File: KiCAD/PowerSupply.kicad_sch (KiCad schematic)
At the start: 63 parts, among them U10 TPS7A39, U11 GM1200, U7 ADP5070ACPZ-R7, U8 TPS7A2033DQN, U9 TPS7A2033DQN

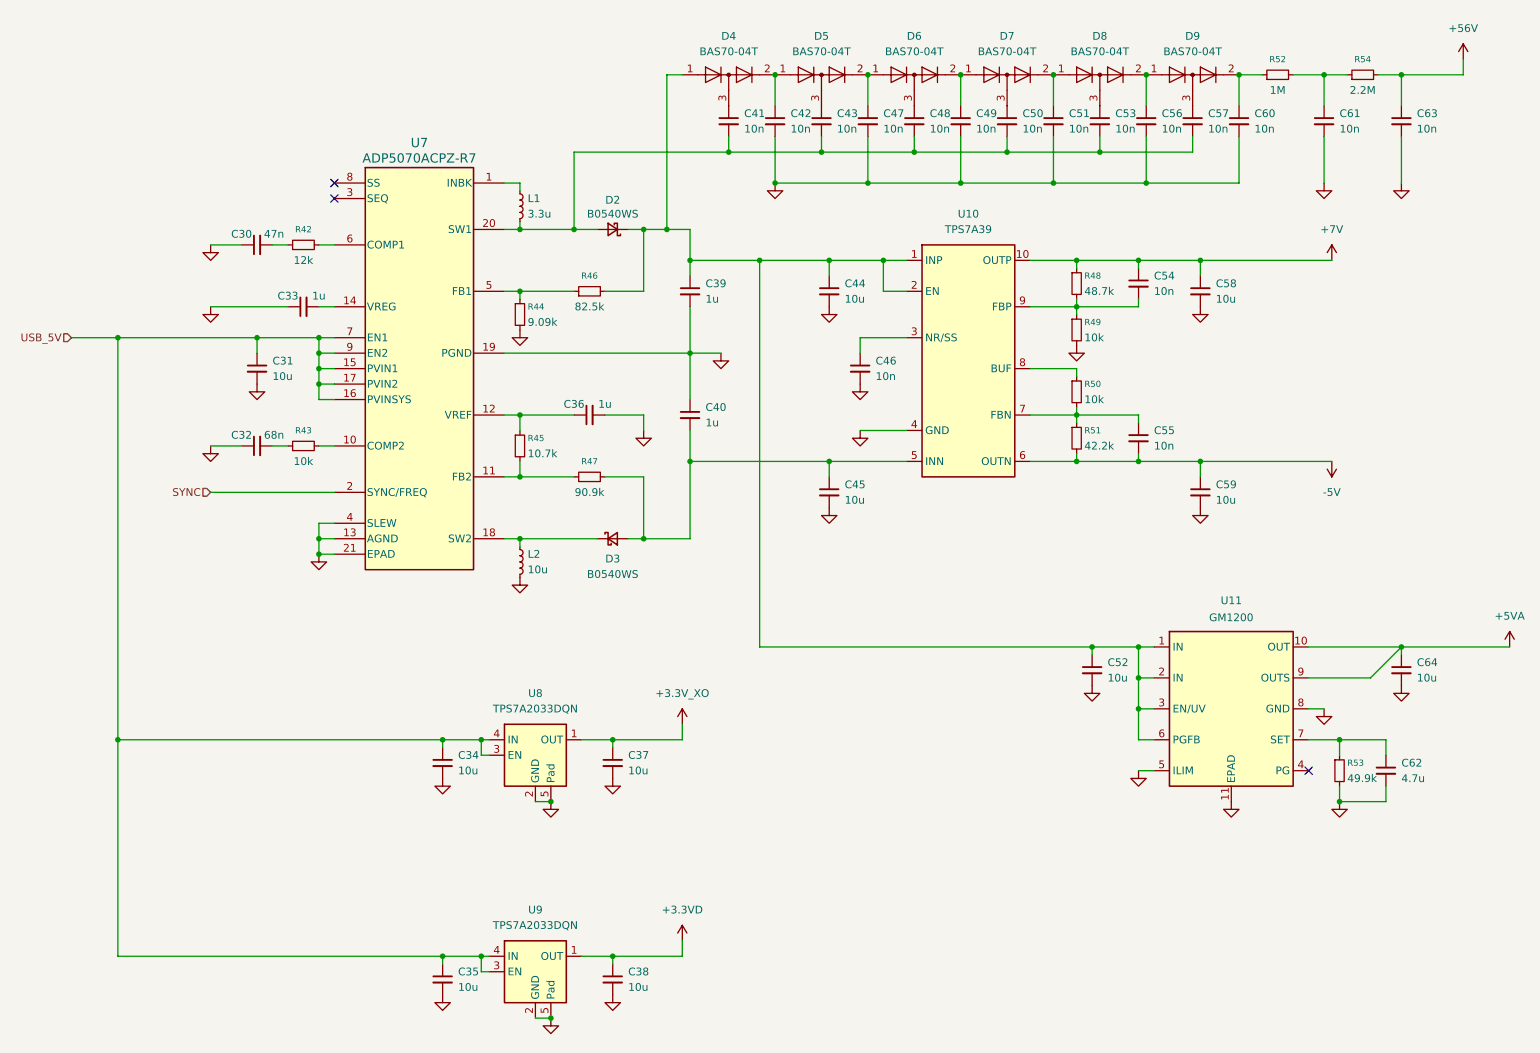
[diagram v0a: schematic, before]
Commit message: 初步layout
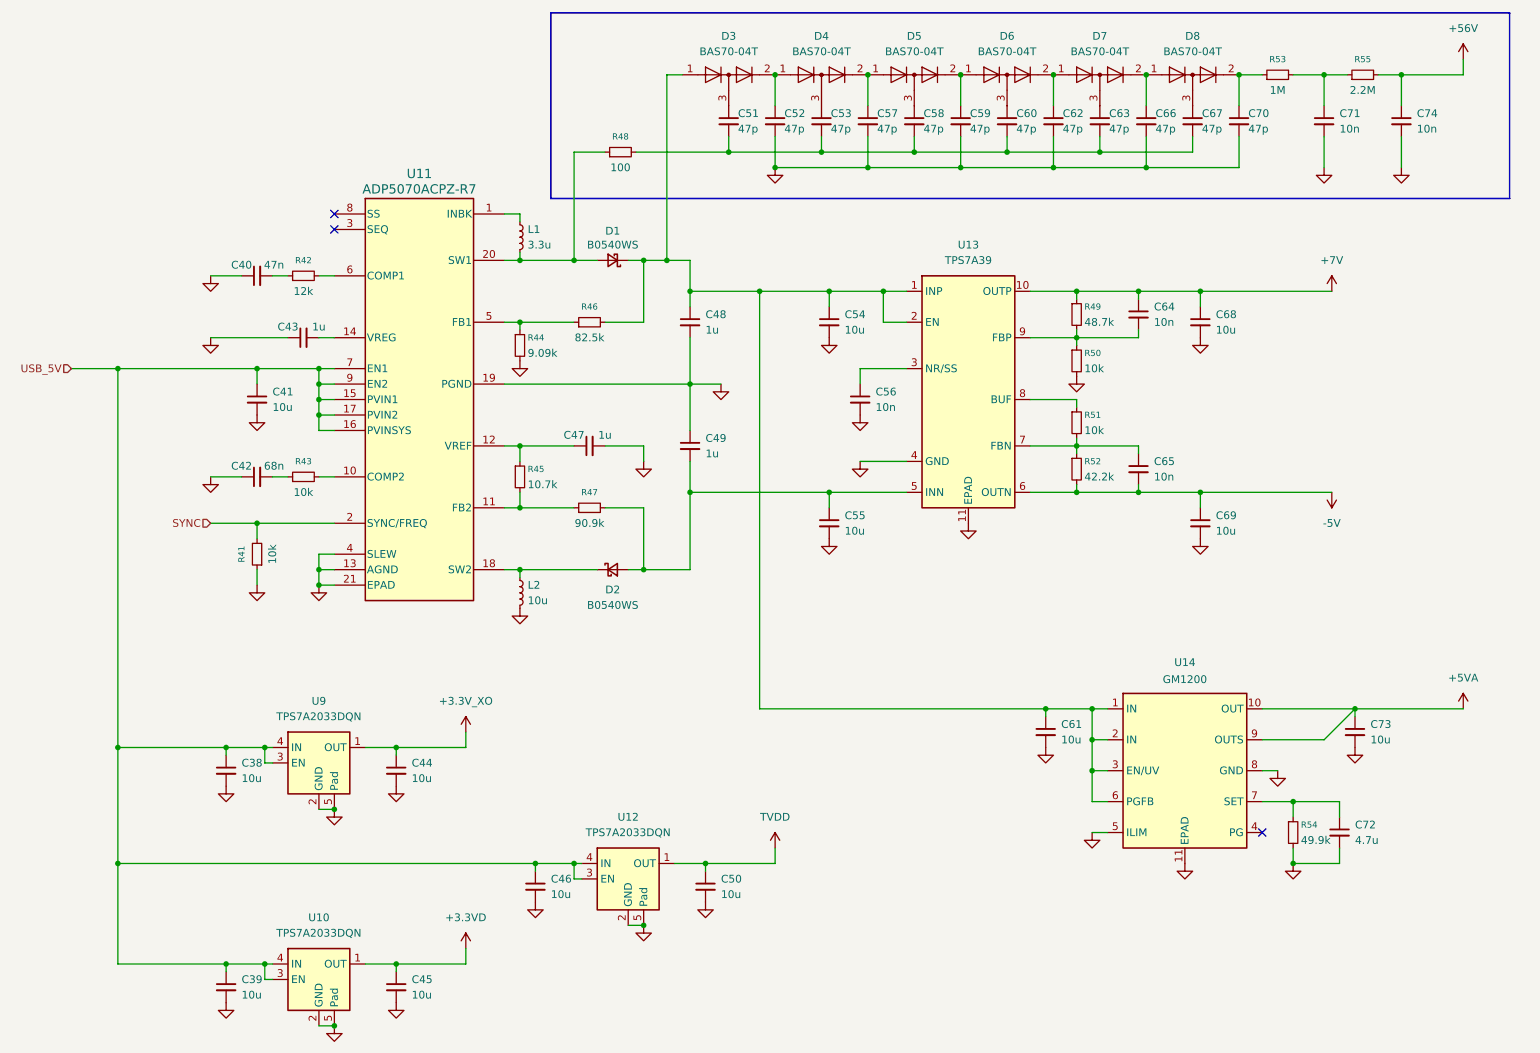
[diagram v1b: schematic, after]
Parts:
- added C46, C50: 10u, Capacitor_SMD:C_0603_1608Metric, symbol Device:C_Small
- added R41: 10k, Resistor_SMD:R_0402_1005Metric, symbol Device:R_Small
- added R48: 100, Resistor_SMD:R_0805_2012Metric, symbol Device:R_Small
- added U12: TPS7A2033DQN, Package_SON:Texas_X2SON-4_1x1mm_P0.65mm, symbol Regulator_Linear:TPS7A20xxxDQN
- C38: renamed from C34; footprint (none) -> Capacitor_SMD:C_0603_1608Metric
- C39: renamed from C35; footprint (none) -> Capacitor_SMD:C_0603_1608Metric
- C40: renamed from C30; footprint (none) -> Capacitor_SMD:C_0402_1005Metric
- C41: renamed from C31; footprint (none) -> Capacitor_SMD:C_0805_2012Metric
- C42: renamed from C32; footprint (none) -> Capacitor_SMD:C_0402_1005Metric
- C43: renamed from C33; footprint (none) -> Capacitor_SMD:C_0402_1005Metric
- C44: renamed from C37; footprint (none) -> Capacitor_SMD:C_0603_1608Metric
- C45: renamed from C38; footprint (none) -> Capacitor_SMD:C_0603_1608Metric
- C47: renamed from C36; footprint (none) -> Capacitor_SMD:C_0402_1005Metric
- C48: renamed from C39; footprint (none) -> Capacitor_SMD:C_0603_1608Metric
- C49: renamed from C40; footprint (none) -> Capacitor_SMD:C_0603_1608Metric
- C51: renamed from C41; value 10n -> 47p; footprint (none) -> Capacitor_SMD:C_0603_1608Metric
- C52: renamed from C42; value 10n -> 47p; footprint (none) -> Capacitor_SMD:C_0603_1608Metric
- C53: renamed from C43; value 10n -> 47p; footprint (none) -> Capacitor_SMD:C_0603_1608Metric
- C54: renamed from C44; footprint (none) -> Capacitor_SMD:C_0603_1608Metric
- C55: renamed from C45; footprint (none) -> Capacitor_SMD:C_0603_1608Metric
- C56: renamed from C46; footprint (none) -> Capacitor_SMD:C_0402_1005Metric
- C57: renamed from C47; value 10n -> 47p; footprint (none) -> Capacitor_SMD:C_0603_1608Metric
- C58: renamed from C48; value 10n -> 47p; footprint (none) -> Capacitor_SMD:C_0603_1608Metric
- C59: renamed from C49; value 10n -> 47p; footprint (none) -> Capacitor_SMD:C_0603_1608Metric
- C60: renamed from C50; value 10n -> 47p; footprint (none) -> Capacitor_SMD:C_0603_1608Metric
- C61: renamed from C52; footprint (none) -> Capacitor_SMD:C_0603_1608Metric
- C62: renamed from C51; value 10n -> 47p; footprint (none) -> Capacitor_SMD:C_0603_1608Metric
- C63: renamed from C53; value 10n -> 47p; footprint (none) -> Capacitor_SMD:C_0603_1608Metric
- C64: renamed from C54; footprint (none) -> Capacitor_SMD:C_0402_1005Metric
- C65: renamed from C55; footprint (none) -> Capacitor_SMD:C_0402_1005Metric
- C66: renamed from C56; value 10n -> 47p; footprint (none) -> Capacitor_SMD:C_0603_1608Metric
- C67: renamed from C57; value 10n -> 47p; footprint (none) -> Capacitor_SMD:C_0603_1608Metric
- C68: renamed from C58; footprint (none) -> Capacitor_SMD:C_0603_1608Metric
- C69: renamed from C59; footprint (none) -> Capacitor_SMD:C_0603_1608Metric
- C70: renamed from C60; value 10n -> 47p; footprint (none) -> Capacitor_SMD:C_0603_1608Metric
- C71: renamed from C61; footprint (none) -> Capacitor_SMD:C_0603_1608Metric
- C72: renamed from C62; footprint (none) -> Capacitor_SMD:C_0603_1608Metric
- C73: renamed from C64; footprint (none) -> Capacitor_SMD:C_0603_1608Metric
- C74: renamed from C63; footprint (none) -> Capacitor_SMD:C_0603_1608Metric
- L1, L2: footprint (none) -> SPM4020T:IND_SPM4020_TDK
- R42, R43, R44, R45, R46, R47: footprint (none) -> Resistor_SMD:R_0402_1005Metric
- R49: renamed from R48; footprint (none) -> Resistor_SMD:R_0402_1005Metric
- R50: renamed from R49; footprint (none) -> Resistor_SMD:R_0402_1005Metric
- R51: renamed from R50; footprint (none) -> Resistor_SMD:R_0402_1005Metric
- R52: renamed from R51; footprint (none) -> Resistor_SMD:R_0402_1005Metric
- R53: renamed from R52; footprint (none) -> Resistor_SMD:R_0805_2012Metric
- R54: renamed from R53; footprint (none) -> Resistor_SMD:R_0402_1005Metric
- R55: renamed from R54; footprint (none) -> Resistor_SMD:R_0805_2012Metric
- U11: renamed from U7; footprint CP-20-8_ADI -> Package_DFN_QFN:QFN-20-1EP_4x4mm_P0.5mm_EP2.6x2.6mm_ThermalVias
- U14: renamed from U11; footprint (none) -> Package_DFN_QFN:DFN-10-1EP_3x3mm_P0.5mm_EP1.65x2.38mm_ThermalVias
- renumbered D2 to D1, D3 to D2, D4 to D3, D5 to D4, D6 to D5, D7 to D6, D8 to D7, D9 to D8, U9 to U10, U10 to U13, U8 to U9
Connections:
- net GND: now also U13.11 (EPAD), C46.2, C50.2, R41.1, U12.2 (GND), U12.5 (Pad)
- net SYNC: now also R41.2
- net USB_5V: now also C46.1, U12.3 (EN), U12.4 (IN)
- net at C51.2, C53.2, C58.2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: now also R48.2; no longer D1.2 (A), L1.2, U11.20 (SW1)
- new net: D1.2 (A), L1.2, R48.1, U11.20 (SW1)
- new net TVDD: C50.1, U12.1 (OUT)
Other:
- moved on the sheet: C38, C39, C40, C41, C42, C43, C44, C45, C47, C48, C49, C54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
